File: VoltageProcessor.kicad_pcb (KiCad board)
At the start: 2 copper layers, 25.4 x 100 mm, 29 parts, among them J1 PJ301M-12, J2 PJ301M-12, J3 Eurorack power, J4 PJ301M-12, J5 PJ301M-12, U1 TL074

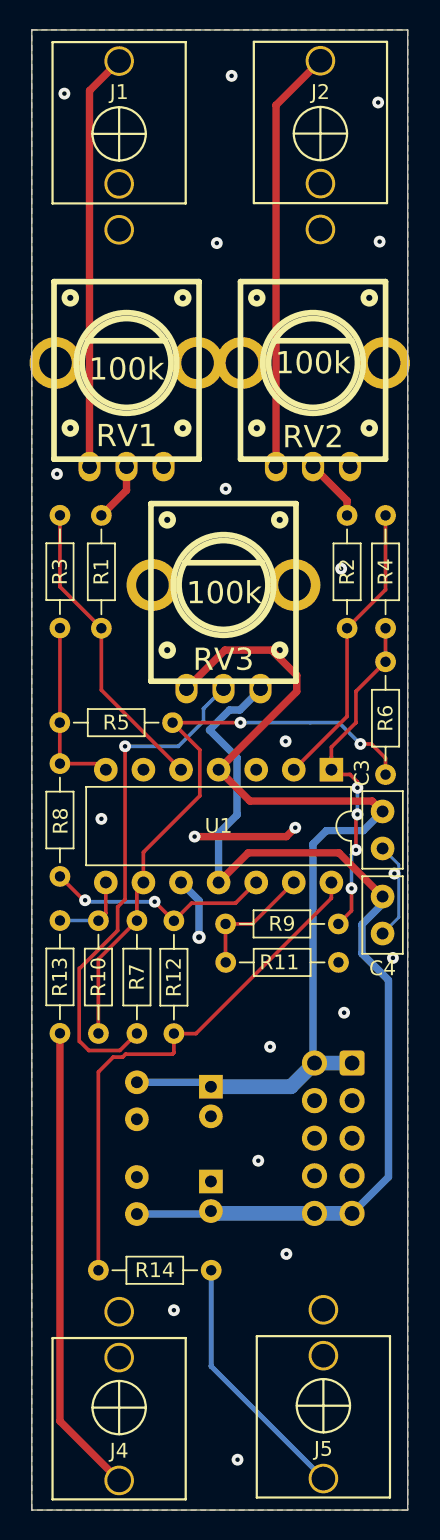
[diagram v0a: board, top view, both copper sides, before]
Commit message: Remove all tracks
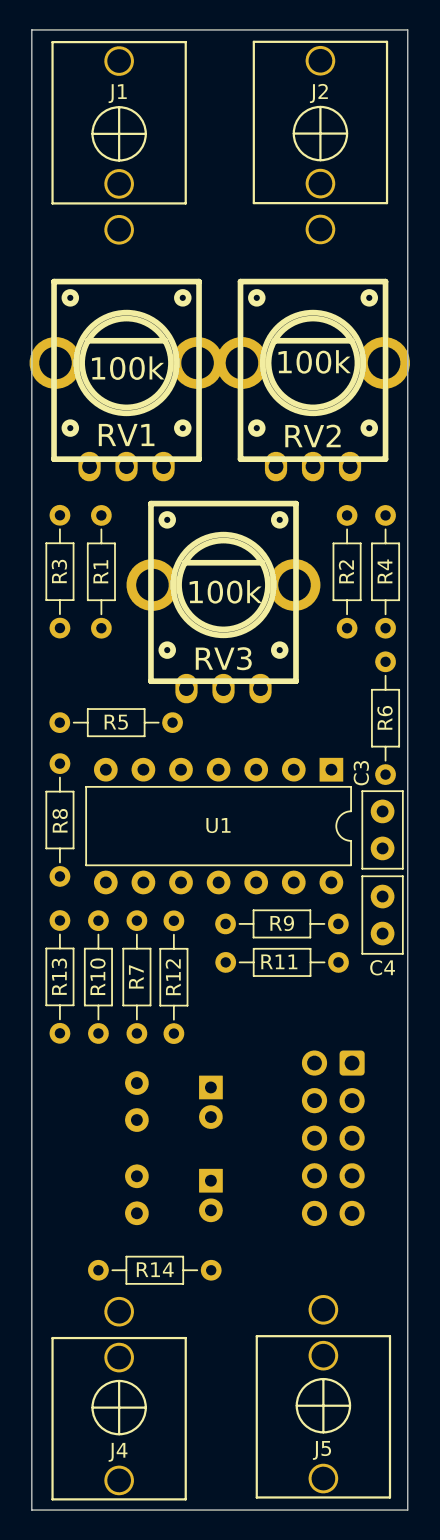
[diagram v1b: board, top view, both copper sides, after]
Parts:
- moved C6 6.35 mm to (106.9, 128.2)
- moved C1 6.35 mm to (101.9, 134.2)
- moved C2 6.35 mm to (101.9, 127.9)
- moved C5 6.35 mm to (106.9, 134.5)
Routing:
- net -12V: track 67.8 -> 0.00 mm
- net +12V: track 66.7 -> 0.00 mm
- net Net-(U1C--): track 41.2 -> 0.00 mm, vias 2 -> 0
- net GND: track 38.5 -> 0.00 mm, vias 21 -> 0
- net Net-(R12-Pad2): track 35.8 -> 0.00 mm
- net Net-(R7-Pad1): track 34.6 -> 0.00 mm, vias 1 -> 0
- net Net-(J4-Pad3): track 31.9 -> 0.00 mm
- net Net-(J2-Pad3): track 28.7 -> 0.00 mm
- net Net-(J1-Pad3): track 28.2 -> 0.00 mm
- net Net-(R4-Pad2): track 24.3 -> 0.00 mm, vias 4 -> 0
- net Net-(U1A--): track 19.7 -> 0.00 mm
- net Net-(J5-Pad3): track 17.2 -> 0.00 mm
- net Net-(U1D-+): track 15.8 -> 0.00 mm, vias 2 -> 0
- net Net-(R3-Pad2): track 12.4 -> 0.00 mm
- net Net-(U1D--): track 8.37 -> 0.00 mm
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- removed copper zone on B.Cu, net GND
- removed copper zone on F.Cu, net GND
